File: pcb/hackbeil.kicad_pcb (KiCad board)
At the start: 2 copper layers, 138.5 x 116.3 mm, 71 parts

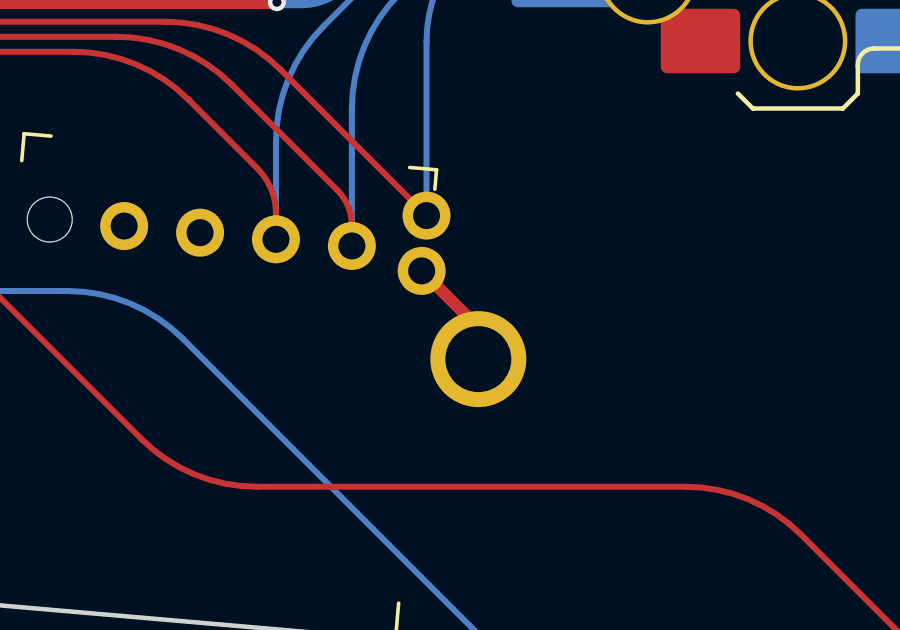
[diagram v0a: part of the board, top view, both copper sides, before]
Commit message: Final routing and top plates
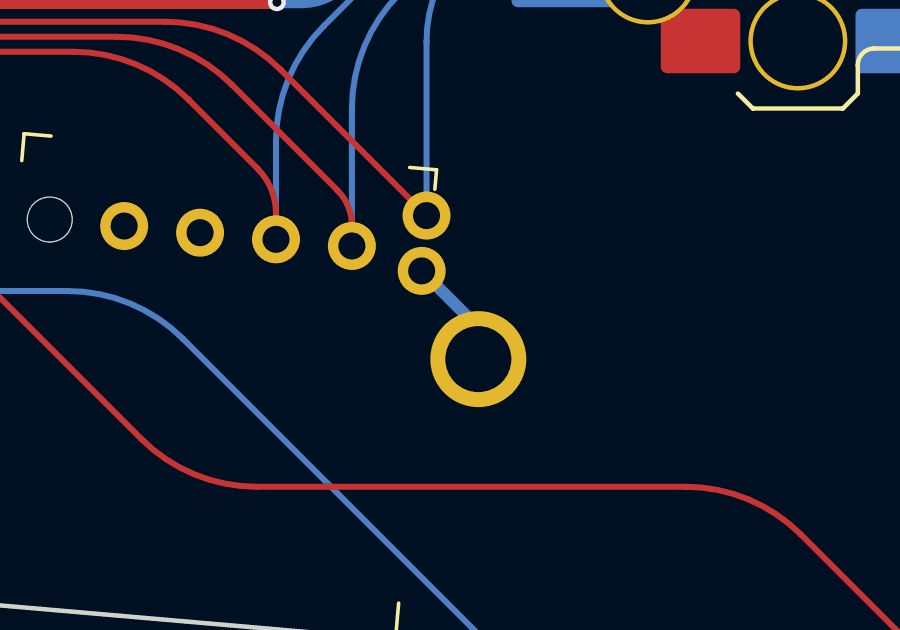
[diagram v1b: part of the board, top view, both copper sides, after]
